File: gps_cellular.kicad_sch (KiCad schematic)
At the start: 46 parts, among them IC1 SGECL01-01-1000, J1 RECE.20279.001E.01, J2 RECE.20279.001E.01, J3 78800-0001, Q1 BC847CE6327HTSA1, Q2 BC847CE6327HTSA1, U2 LENA-R8001M10-00C

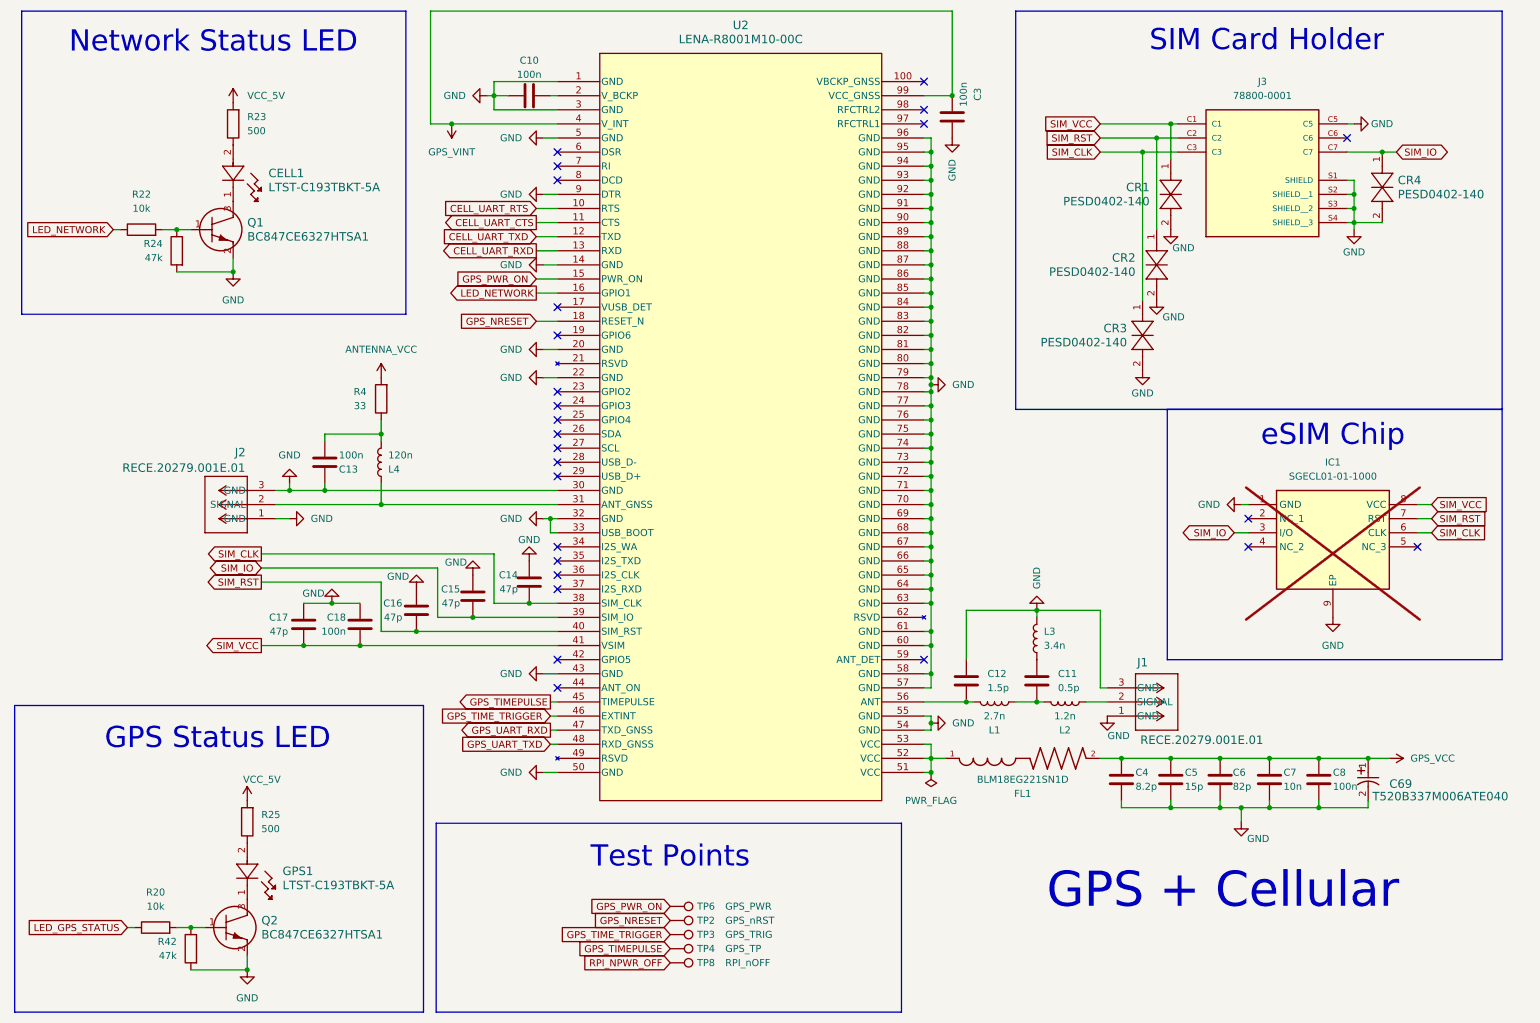
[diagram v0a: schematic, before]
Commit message: Update for RevB
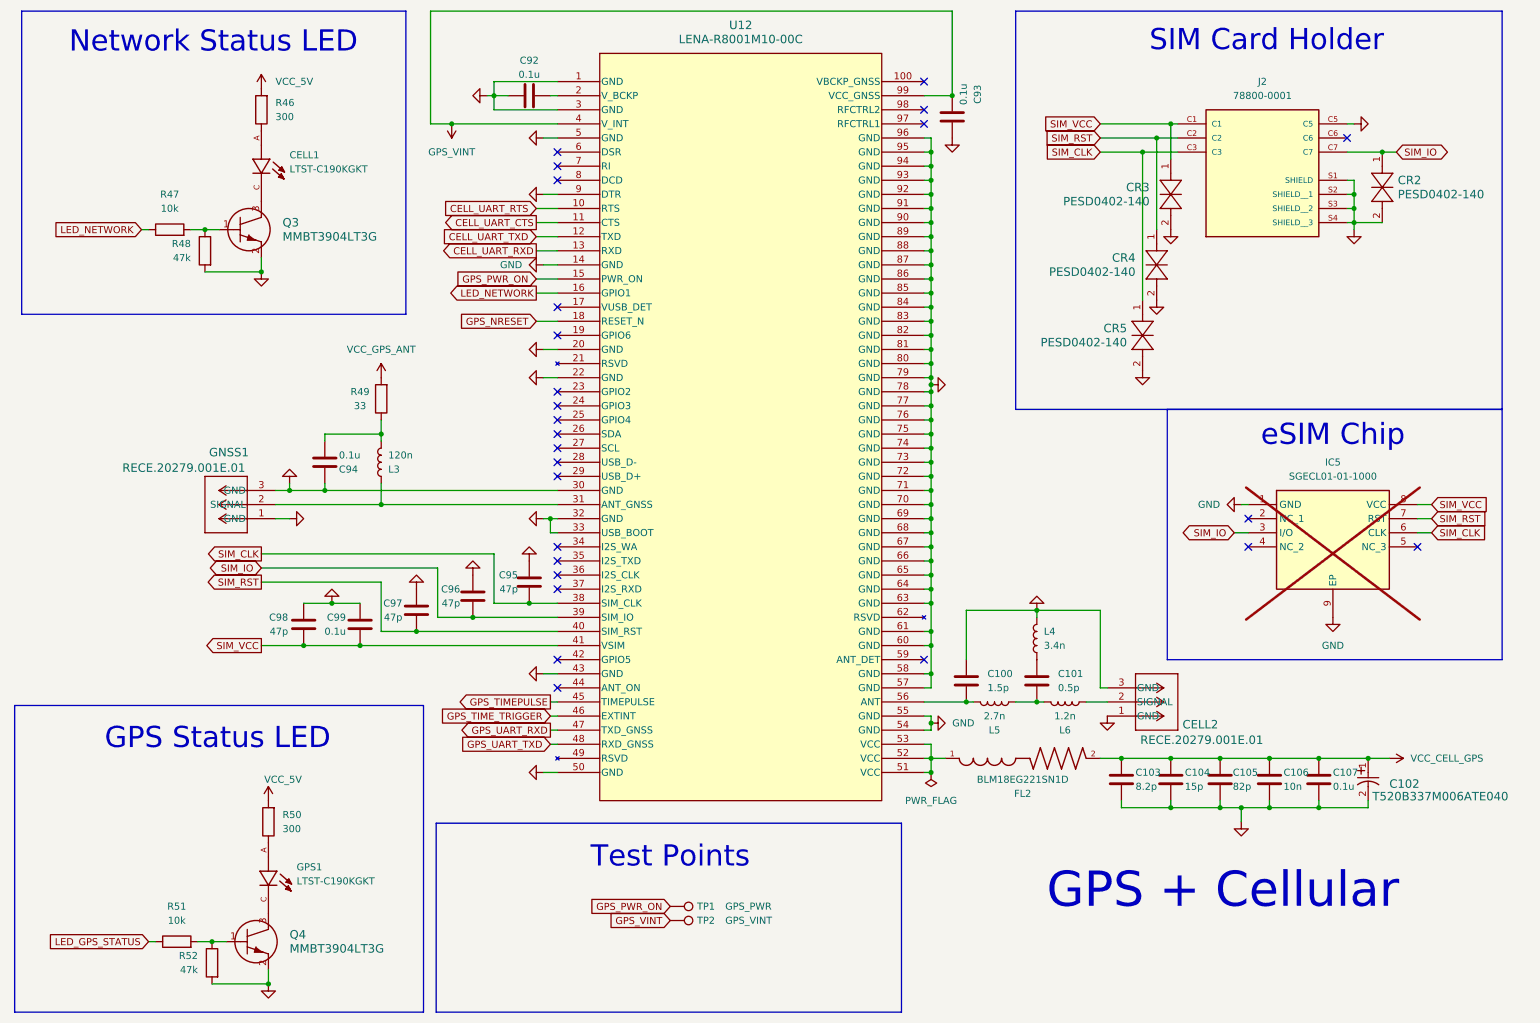
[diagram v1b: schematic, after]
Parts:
- removed CELL1, GPS1: LTST-C193TBKT-5A, CivicAlert:LTST-C193TBKT-5A, symbol LTST-C193TBKT-5A:LTST-C193TBKT-5A
- removed Q1, Q2: BC847CE6327HTSA1, CivicAlert:BC847CE6327HTSA1, symbol BC847CE6327HTSA1:BC847CE6327HTSA1
- removed TP2: GPS_nRST, TestPoint:TestPoint_THTPad_D1.0mm_Drill0.5mm, symbol Connector:TestPoint
- removed TP4: GPS_TP, TestPoint:TestPoint_THTPad_D1.0mm_Drill0.5mm, symbol Connector:TestPoint
- removed TP8: RPI_nOFF, TestPoint:TestPoint_THTPad_D1.0mm_Drill0.5mm, symbol Connector:TestPoint
- added CELL1, GPS1: LTST-C190KGKT, CivicAlert:LTST-C190KGKT, symbol LTST-C190KGKT:LTST-C190KGKT
- added Q3, Q4: MMBT3904LT3G, CivicAlert:MMBT3904LT3G, symbol MMBT3904LT3G:BC847CE6327HTSA1
- C100: renamed from C12; MANUFACTURER Murata -> (none); MPN GRT1555C1H1R5CA02J -> (none); Manufacturer (none) -> Murata
- C101: renamed from C11; MANUFACTURER Murata -> (none); MPN GJM1555C1HR50WB01 -> (none); Manufacturer (none) -> Murata
- C102: renamed from C69; MANUFACTURER KEMET -> (none); MPN T520B337M006ATE040 -> (none); Manufacturer (none) -> KEMET
- C103: renamed from C4; MANUFACTURER Murata -> (none); MPN GRT1555C1H8R2DA02D -> (none); Manufacturer (none) -> Murata
- C104: renamed from C5; MANUFACTURER Murata -> (none); MPN GRT1555C1H150JA02J -> (none); Manufacturer (none) -> Murata
- C105: renamed from C6; MANUFACTURER Murata -> (none); MPN GRT1555C1H820FA02D -> (none); Manufacturer (none) -> Murata
- C106: renamed from C7; MANUFACTURER Murata -> (none); MPN GCM155R71H103KA55D -> (none); Manufacturer (none) -> Murata
- C107: renamed from C8; value 100n -> 0.1u; MANUFACTURER Murata -> (none); MPN GRT155R71H104KE01D -> (none); Manufacturer (none) -> Murata
- C92: renamed from C10; value 100n -> 0.1u; MANUFACTURER Murata -> (none); MPN GRT155R71H104KE01D -> (none); Manufacturer (none) -> Murata
- C93: renamed from C3; value 100n -> 0.1u; MANUFACTURER Murata -> (none); MPN GRT155R71H104KE01D -> (none); Manufacturer (none) -> Murata
- C94: renamed from C13; value 100n -> 0.1u; MANUFACTURER Murata -> (none); MPN GRT155R71H104KE01D -> (none); Manufacturer (none) -> Murata
- C95: renamed from C14; MANUFACTURER Murata -> (none); MPN GRT1555C1H470JA02J -> (none); Manufacturer (none) -> Murata
- C96: renamed from C15; MANUFACTURER Murata -> (none); MPN GRT1555C1H470JA02J -> (none); Manufacturer (none) -> Murata
- C97: renamed from C16; MANUFACTURER Murata -> (none); MPN GRT1555C1H470JA02J -> (none); Manufacturer (none) -> Murata
- C98: renamed from C17; MANUFACTURER Murata -> (none); MPN GRT1555C1H470JA02J -> (none); Manufacturer (none) -> Murata
- C99: renamed from C18; value 100n -> 0.1u; MANUFACTURER Murata -> (none); MPN GRT155R71H104KE01D -> (none); Manufacturer (none) -> Murata
- CELL2: renamed from J1; MANUFACTURER Taoglas -> (none); MPN RECE.20279.001E.01 -> (none); Manufacturer (none) -> Taoglas
- CR2: renamed from CR4; MANUFACTURER Littelfuse -> (none); MPN PESD0402-140 -> (none); Manufacturer (none) -> Littelfuse
- CR3: renamed from CR1; MANUFACTURER Littelfuse -> (none); MPN PESD0402-140 -> (none); Manufacturer (none) -> Littelfuse
- CR4: renamed from CR2; MANUFACTURER Littelfuse -> (none); MPN PESD0402-140 -> (none); Manufacturer (none) -> Littelfuse
- CR5: renamed from CR3; MANUFACTURER Littelfuse -> (none); MPN PESD0402-140 -> (none); Manufacturer (none) -> Littelfuse
- FL2: renamed from FL1; MANUFACTURER Murata -> (none); MPN BLM18EG221SN1D -> (none); Manufacturer (none) -> Murata
- GNSS1: renamed from J2; MANUFACTURER Taoglas -> (none); MPN RECE.20279.001E.01 -> (none); Manufacturer (none) -> Taoglas
- J2: renamed from J3; MANUFACTURER Molex -> (none); MAXIMUM_PACKAGE_HEIGHT 1.6 mm -> (none); MPN 78800-0001 -> (none); Manufacturer (none) -> Molex; PARTREV A -> (none); STANDARD Manufacturer Recommendations -> (none)
- L3: renamed from L4; MANUFACTURER Murata -> (none); MPN LQW15ANR12J00 -> (none); Manufacturer (none) -> Murata
- L4: renamed from L3; MANUFACTURER Murata -> (none); MPN LQG15WZ3N4S02D -> (none); Manufacturer (none) -> Murata
- L5: renamed from L1; MANUFACTURER Murata -> (none); MPN LQG15HH2N7B02 -> (none); Manufacturer (none) -> Murata
- L6: renamed from L2; MANUFACTURER Murata -> (none); MPN LQG15HH1N2B02 -> (none); Manufacturer (none) -> Murata
- R46: renamed from R23; value 500 -> 300
- R50: renamed from R25; value 500 -> 300
- TP2: renamed from TP3; value GPS_TRIG -> GPS_VINT
- U12: renamed from U2; MANUFACTURER u-blox -> (none); MPN LENA-R8001M10-00C -> (none); Manufacturer (none) -> u-blox
- renumbered IC1 to IC5, R22 to R47, R24 to R48, R4 to R49, R20 to R51, R42 to R52, TP6 to TP1
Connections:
- net GND: now also Q3.2, Q4.2
- net GPS_TIME_TRIGGER: no longer TP2.1
- net GPS_VINT: now also TP2.1
- net at R50.1: now also GPS1.A
- net at R46.1: now also CELL1.A
- net at R51.2, R52.1: now also Q4.1
- net at R47.2, R48.1: now also Q3.1
- net ANTENNA_VCC renamed VCC_GPS_ANT
- net GPS_VCC renamed VCC_CELL_GPS
- new net: CELL1.C, Q3.3
- new net: GPS1.C, Q4.3
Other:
- moved on the sheet: R46, R47, R48, R50, R51, R52, TP2

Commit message: Finalize RevB
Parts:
- C100: MPN (none) -> GRT1555C1H1R5CA02J
- C101: MPN (none) -> GJM1555C1HR50WB01D
- C102: MPN (none) -> T520B337M006ATE040
- C103: MPN (none) -> GRM1555C1E8R2CA01D
- C104: MPN (none) -> GRT1555C1H150JA02J
- C105: MPN (none) -> GRT1555C1H820FA02D
- C106: MPN (none) -> GCM155R71H103KA55D
- C107, C92, C93, C94, C99: MPN (none) -> GRM155R71C104KA88J
- C95, C96, C97, C98: MPN (none) -> GRT1555C1H470JA02J
- CELL1, GPS1: MPN (none) -> LTST-C190KGKT
- CELL2, GNSS1: MPN (none) -> RECE.20279.001E.01
- CR2, CR3, CR4, CR5: MPN (none) -> PESD0402-140
- FL2: MPN (none) -> BLM18EG221SN1D
- IC5: Height 0.8 -> (none); Manufacturer_Name Soracom -> (none); Manufacturer_Part_Number SGECL01-01-1000 -> (none); Mouser Part Number 432-SGECL01-01-1000 -> (none); Mouser Price/Stock https://www.mouser.co.uk/ProductDetail/Soracom/SGECL01-01-1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 -> (none)
- J2: MPN (none) -> 0788000001
- L3: MPN (none) -> LQW15ANR12J00
- L4: MPN (none) -> LQG15WZ3N4S02D
- L5: MPN (none) -> LQG15HS2N7B02D
- L6: MPN (none) -> LQG15HS1N2B02D
- Q3, Q4: MPN (none) -> BC847CE6327HTSA1
- U12: MPN (none) -> LENA-R8001M10-00C
